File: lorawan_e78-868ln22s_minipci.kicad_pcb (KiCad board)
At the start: 2 copper layers, 30 x 51 mm, 22 parts, among them Con1 MiniPci, Con2 TC2050-IDC-NL, P1 RF2-03E-T-00-50-G, U1 DS18B20U, U2 TCN75A, U8 IP4220CZ6

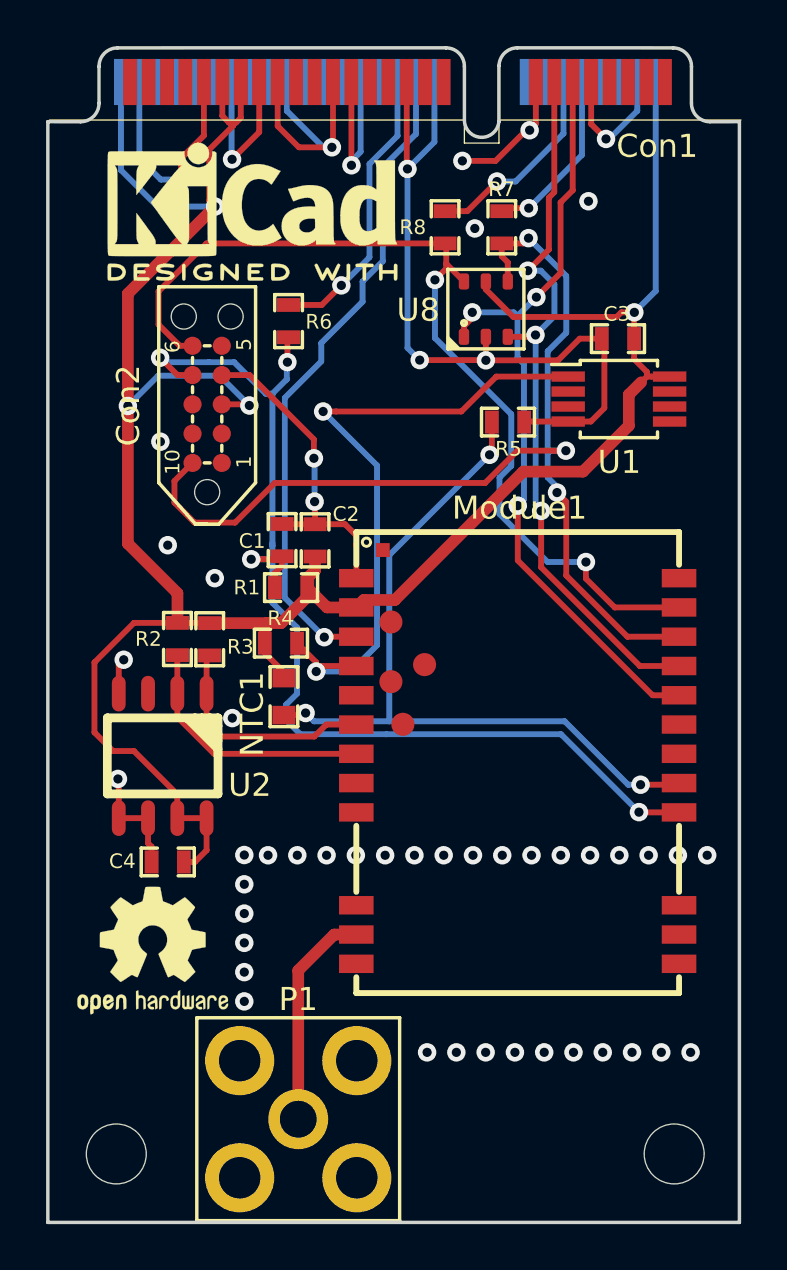
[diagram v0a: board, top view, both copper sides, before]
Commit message: Corrected project
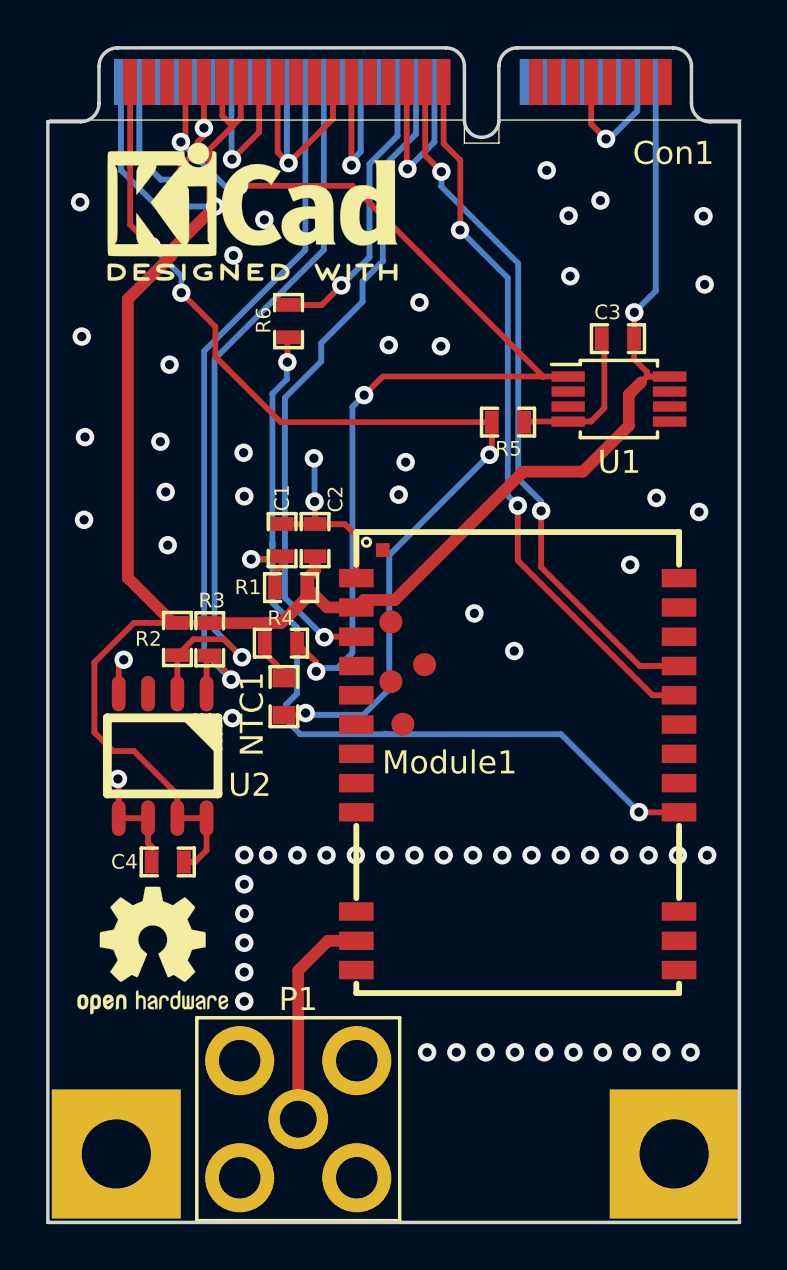
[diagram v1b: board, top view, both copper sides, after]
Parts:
- removed Con2: TC2050-IDC-NL, Tag_Connectors:TC2050-IDC-NL
- removed R7, R8: 0R, Resistor_Smd_0603:0R_0603
- removed U8: IP4220CZ6, ESD_Protectors:IP4220CZ6_SOT457
- added REF**: KiCad-Logo2_8mm_SilkScreen, Symbols:KiCad-Logo2_8mm_SilkScreen, B.Cu at (152.7, 93.3)
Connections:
- Con1 pad 10: Net-(Con1-Pad10) -> (no net)
- Con1 pad 11: Net-(Con1-Pad11) -> (no net)
- Con1 pad 12: Net-(Con1-Pad12) -> (no net)
- Con1 pad 13: Net-(Con1-Pad13) -> (no net)
- Con1 pad 17: (no net) -> Net-(Con1-Pad17)
- Con1 pad 19: (no net) -> Net-(Con1-Pad19)
- Con1 pad 30: (no net) -> Net-(Con1-Pad30)
- Con1 pad 32: (no net) -> Net-(Con1-Pad32)
- Con1 pad 45: (no net) -> Net-(Con1-Pad45)
- Con1 pad 51: (no net) -> Net-(Con1-Pad51)
- Module1 pad 17: Net-(Module1-Pad17) -> (no net)
- Module1 pad 20: Net-(Con1-Pad11) -> Net-(Con1-Pad17)
- Module1 pad 21: Net-(Con1-Pad13) -> Net-(Con1-Pad19)
- Module1 pad 22: Net-(Con2-Pad10) -> (no net)
- Module1 pad 23: Net-(Con2-Pad6) -> (no net)
- Module1 pad 4: Net-(Module1-Pad4) -> (no net)
- Module1 pad 6: Net-(Module1-Pad6) -> (no net)
- Module1 pad 7: Net-(Module1-Pad7) -> (no net)
- NTC1 pad 1: Net-(Module1-Pad17) -> Net-(Con1-Pad51)
- R2 pad 2: Net-(Module1-Pad7) -> Net-(Con1-Pad30)
- R3 pad 2: Net-(Module1-Pad6) -> Net-(Con1-Pad32)
- R4 pad 2: Net-(Module1-Pad4) -> Net-(Con1-Pad45)
- R5 pad 1: Net-(Module1-Pad17) -> Net-(Con1-Pad51)
- U1 pad 1: Net-(Module1-Pad4) -> Net-(Con1-Pad45)
- U2 pad 1: Net-(Module1-Pad6) -> Net-(Con1-Pad32)
- U2 pad 2: Net-(Module1-Pad7) -> Net-(Con1-Pad30)
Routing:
- net Net-(Con1-Pad45): track 0.00 -> 46.7 mm, vias 0 -> 4
- net Net-(Con2-Pad10): track 46.5 -> 0.00 mm, vias 3 -> 0
- net Net-(Con1-Pad51): track 0.00 -> 45.1 mm, vias 0 -> 4
- net Net-(Con2-Pad6): track 41.1 -> 0.00 mm, vias 2 -> 0
- net Net-(Con1-Pad11): track 34.6 -> 0.00 mm, vias 3 -> 0
- net Net-(Module1-Pad17): track 33.3 -> 0.00 mm, vias 3 -> 0
- net Net-(Con1-Pad30): track 0.00 -> 32.5 mm, vias 0 -> 1
- net Net-(Con1-Pad13): track 31.8 -> 0.00 mm, vias 3 -> 0
- net Net-(Con1-Pad17): track 0.00 -> 31.5 mm, vias 0 -> 2
- net Net-(Con1-Pad32): track 0.00 -> 31.4 mm, vias 0 -> 1
- net Net-(Con1-Pad19): track 0.00 -> 30.9 mm, vias 0 -> 2
- net GND: track 100.9 -> 71.6 mm, vias 52 -> 72
- net Net-(Module1-Pad4): track 28.9 -> 0.00 mm, vias 2 -> 0
- net 3V3: track 119.2 -> 102.7 mm, vias 4 -> 2
- net Net-(Module1-Pad7): track 11.1 -> 0.00 mm
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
